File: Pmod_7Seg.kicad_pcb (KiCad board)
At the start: 2 copper layers, 71.6 x 43.2 mm, 13 parts, among them IC1 TBD62783APG, IC2 TBD62003APG, IC3 OSL60362-LR, J1 Conn_02x06_Counter_Clockwise, J2 Conn_02x06_Counter_Clockwise

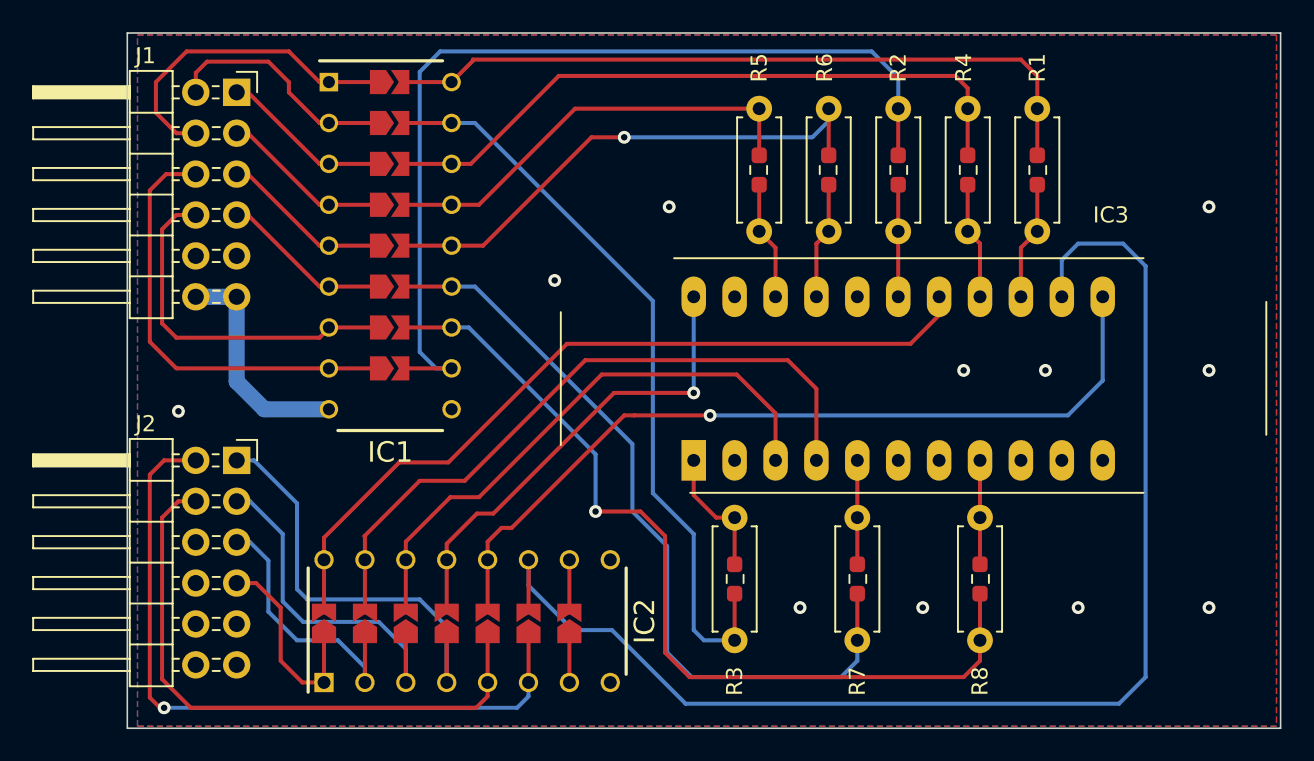
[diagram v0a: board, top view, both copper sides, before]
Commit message: 15
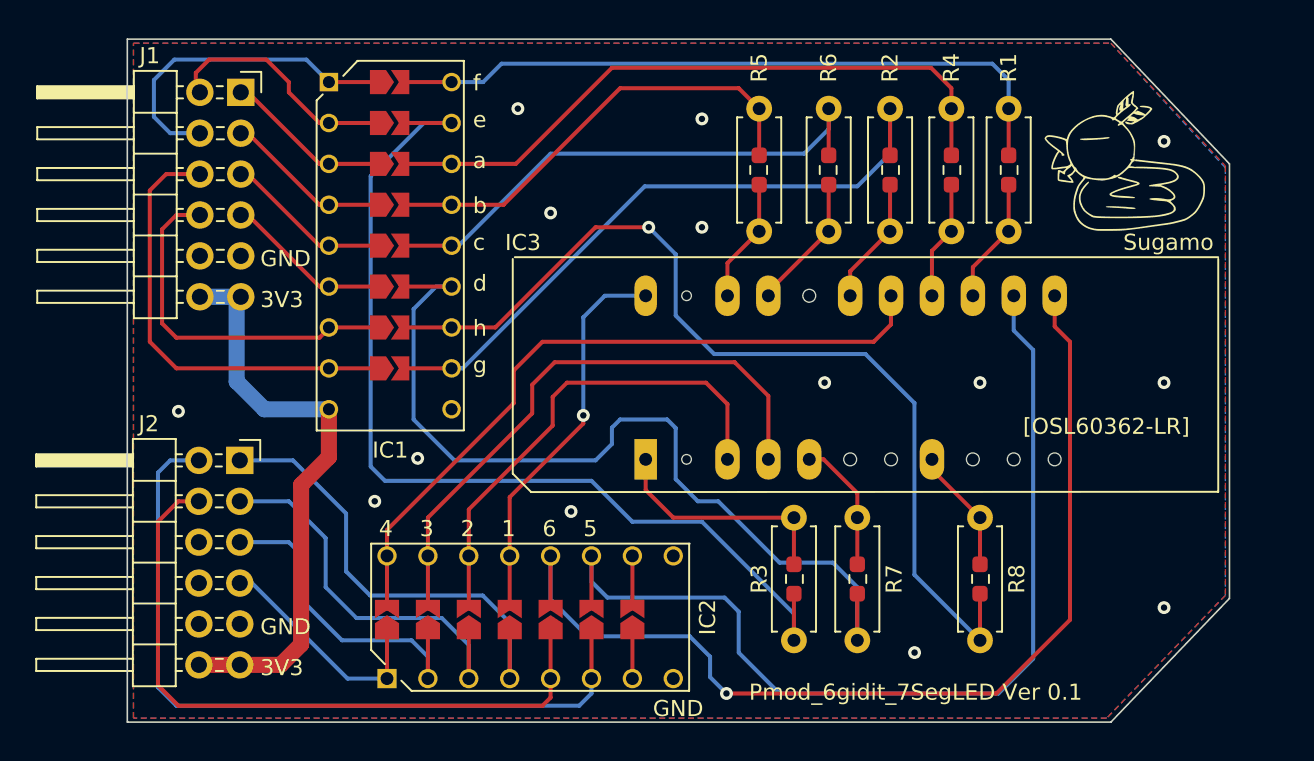
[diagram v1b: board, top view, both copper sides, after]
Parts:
- added G***: LOGO, MyLibrary:logo_kamo_ss, F.Cu at (167.4, 70.4)
- IC3: footprint Library:OSL60362-LR-with-allpin -> MyLibrary:OSL60362-LR-with-allpin
- moved IC2 3.92 mm to (130.6, 98.6)
- moved R3 3.68 mm to (146.9, 100.1)
- moved IC3 2.99 mm to (137.7, 88.8)
- moved R1 1.78 mm to (160.3, 74.7)
- moved R4 1.02 mm to (156.7, 74.7)
- moved R2 0.51 mm to (152.9, 74.7)
- moved J1 0.25 mm to (101.3, 66.0)
- moved J2 0.19 mm to (101.2, 88.9)
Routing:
- net VCC: track 14.2 -> 36.6 mm
- net Net-(DS1-KATHODE_5): track 80.6 -> 60.3 mm
- net Net-(IC1-O8): track 58.7 -> 41.6 mm
- net Net-(IC1-O2): track 47.4 -> 62.2 mm
- net Net-(DS1-KATHODE_6): track 51.6 -> 63.5 mm
- net Net-(DS1-ANODE_E): track 8.18 -> 14.7 mm
- net Net-(IC1-O6): track 49.3 -> 55.6 mm
- net Net-(DS1-KATHODE_3): track 42.2 -> 36.3 mm
- net Net-(DS1-KATHODE_4): track 49.7 -> 43.9 mm
- net Net-(DS1-KATHODE_2): track 35.2 -> 30.2 mm
- net Net-(DS1-KATHODE_1): track 29.1 -> 24.1 mm
- net Net-(J2-Pin_8): track 37.9 -> 42.6 mm
- net Net-(IC1-O7): track 55.8 -> 60.5 mm
- net Net-(J2-Pin_3): track 17.2 -> 21.0 mm
- net Net-(J2-Pin_2): track 22.1 -> 25.2 mm
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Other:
- board size 71.6 x 43.2 mm -> 68.5 x 42.4 mm
- board text added: "1"
- board text added: "2"
- board text added: "3"
- board text added: "3V3"
- board text added: "4"
- board text added: "5"
- board text added: "6"
- board text added: "GND"
- board text added: "Pmod_6gidit_7SegLED Ver 0.1"
- board text added: "Sugamo"
- board text added: "[OSL60362-LR]"
- board text added: "[TBD62003APG]"
- board text added: "[TBD62783APG]"
- board text added: "a"
- board text added: "b"
- board text added: "c"
- board text added: "d"
- board text added: "e"
- board text added: "f"
- board text added: "g"
- board text added: "h"
